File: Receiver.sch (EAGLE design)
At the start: 11 parts, among them IC1 25LC080P, J1 PIC_ICSP_6_PIN, U1 915MHz, U2 DS3234, X1 BU-SMA-V

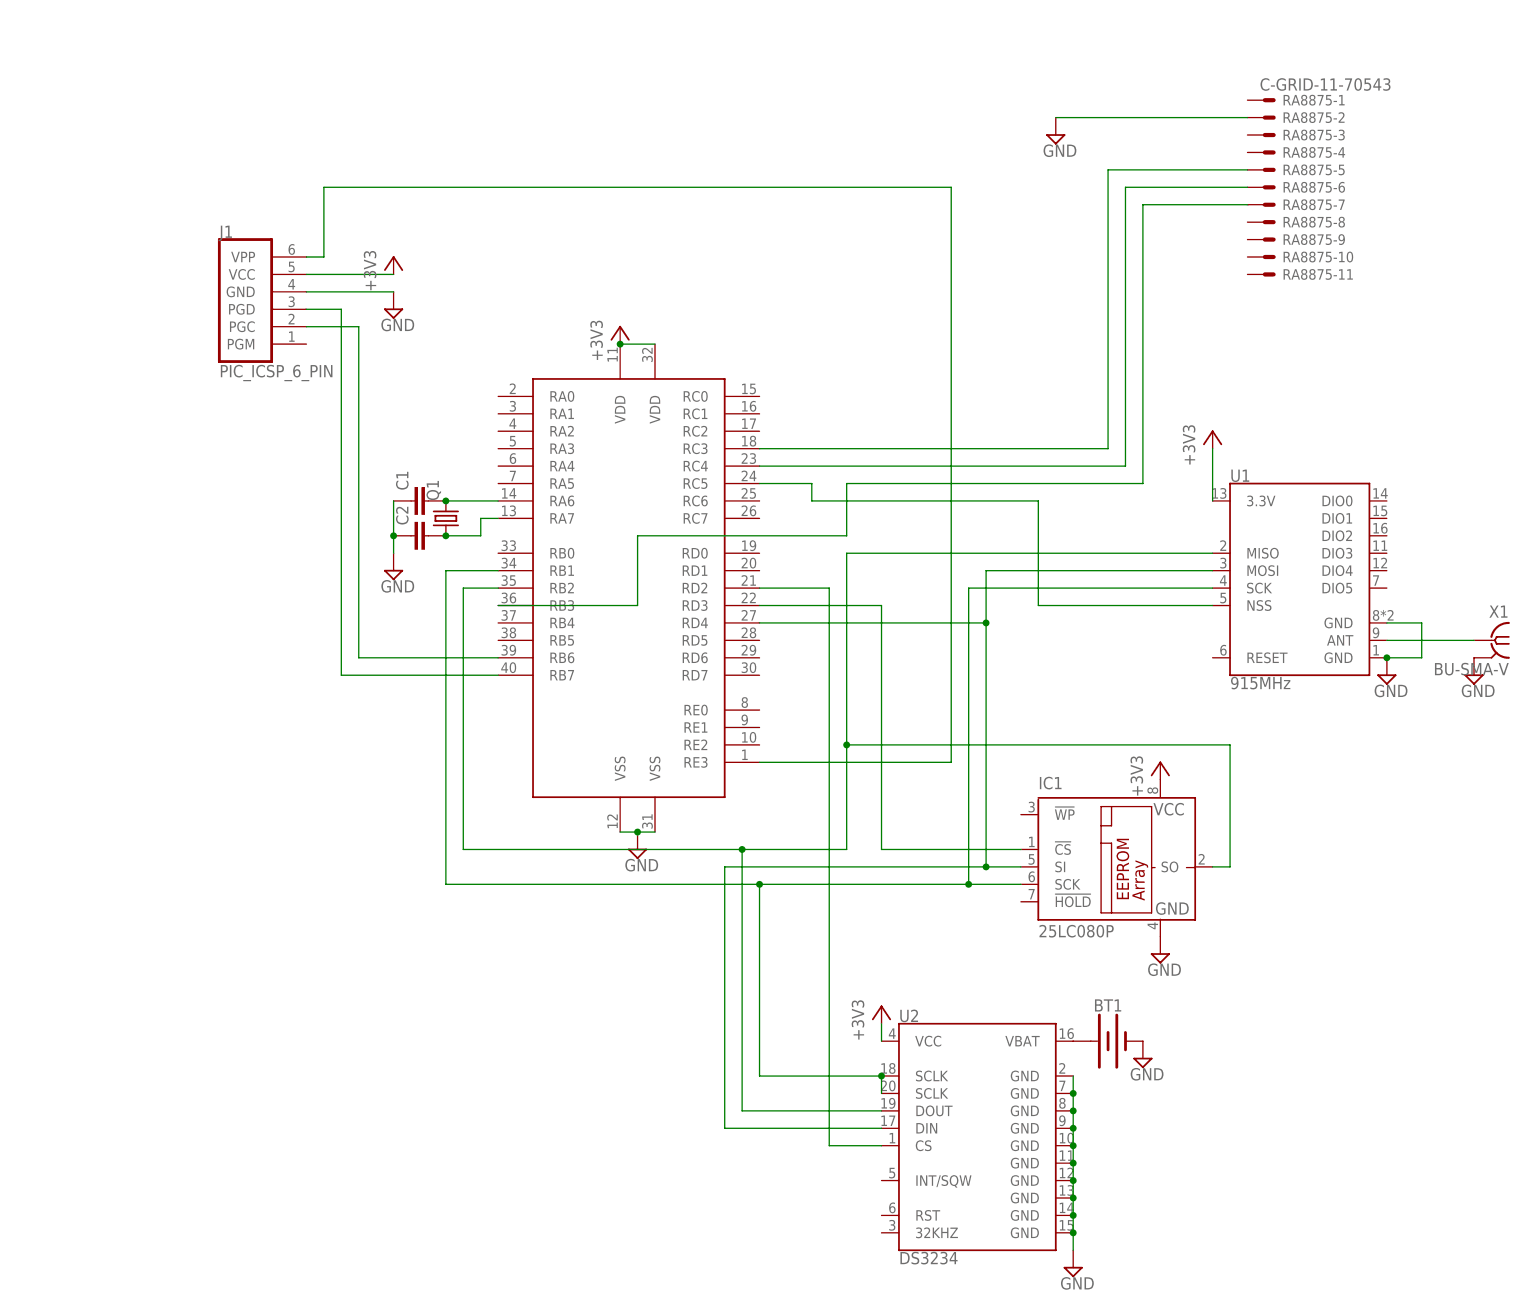
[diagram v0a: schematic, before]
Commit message: Updates
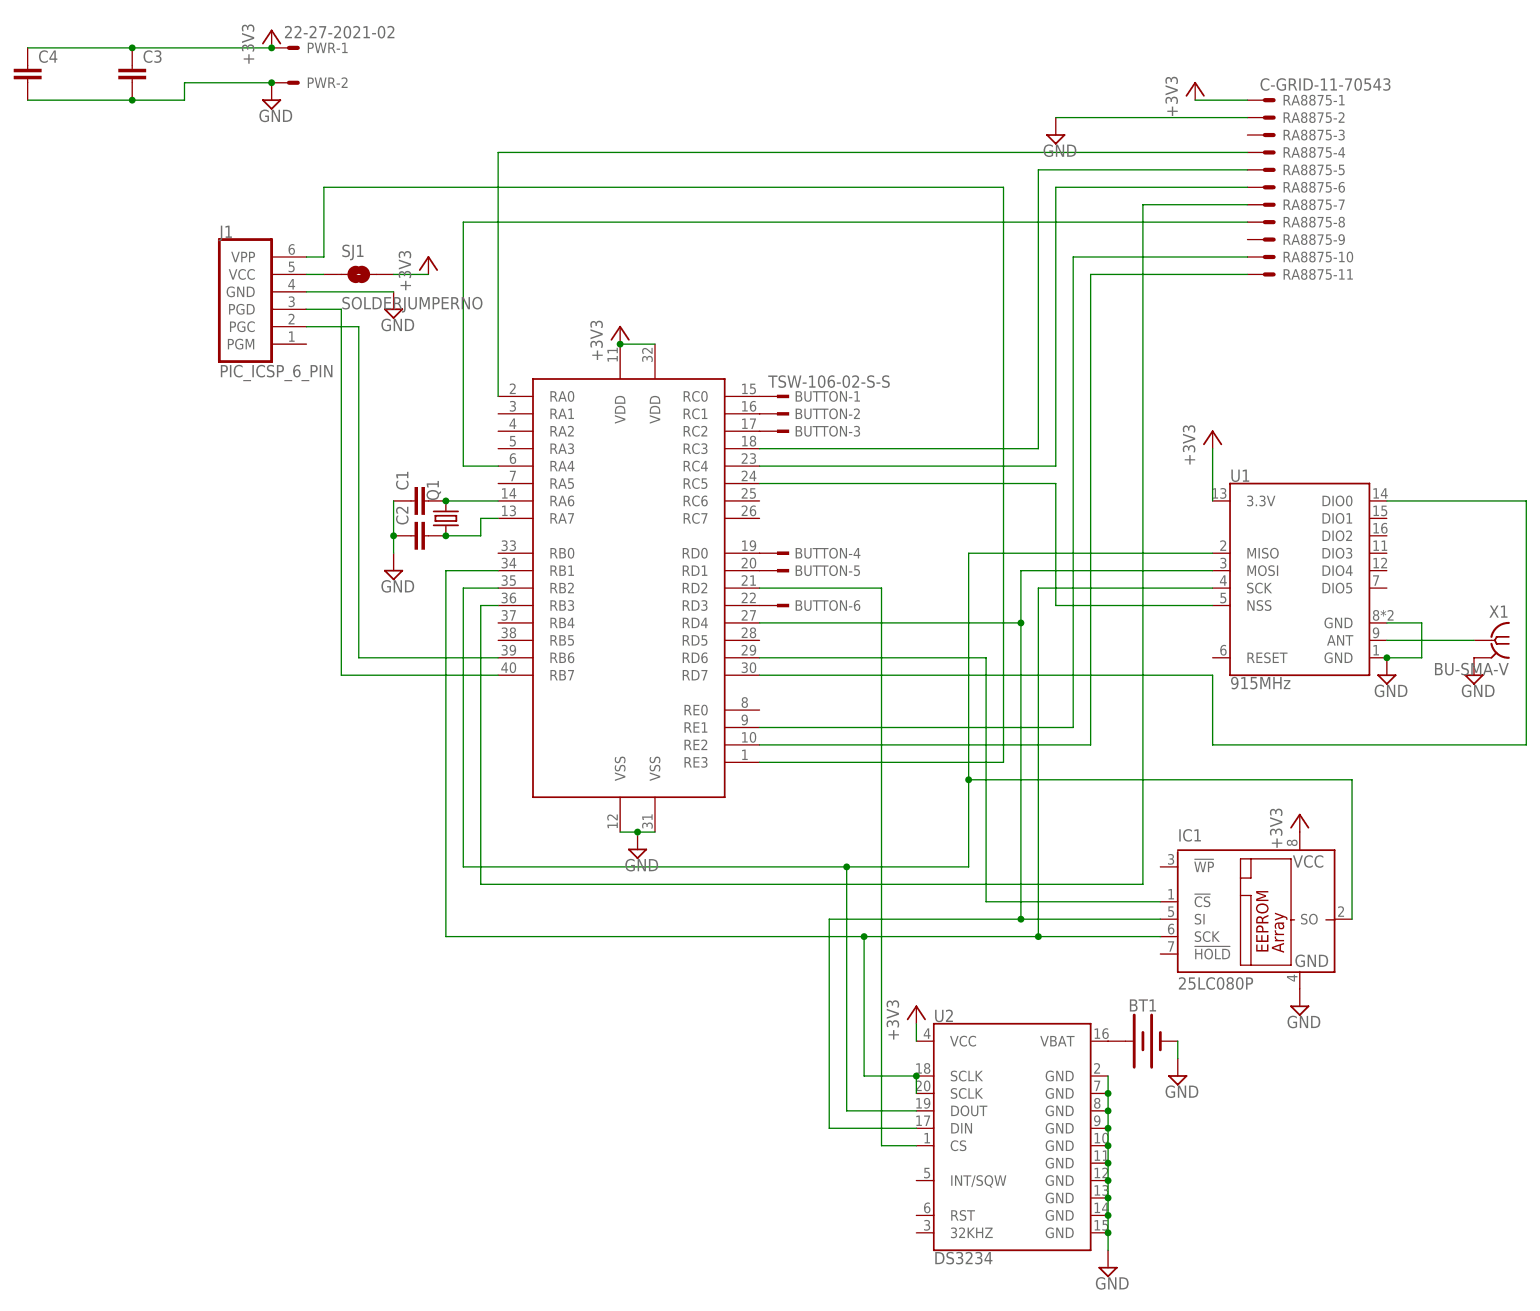
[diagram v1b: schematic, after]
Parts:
- added BUTTON: TSW-106-02-S-S, con-samtec:TSW-106-02-S-S
- added C3, C4: (no value), resistor:C-EU050-025X075
- added PWR: 22-27-2021-02, con-molex:22-27-2021-02
- added SJ1: SOLDERJUMPERNO, SparkFun-Retired:SOLDERJUMPERNO
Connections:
- net N$10 renamed MOSI1
- net N$11 renamed MOSI2
- net N$6 renamed SCK1
- net N$7 renamed MISO1
- net N$8 renamed SCK2
- net N$9 renamed MISO2
- new net N$10: BUTTON-4.1, U$1.RD0
- new net N$11: BUTTON-6.1, U$1.RD3
- new net N$17: RA8875-8.S, U$1.RA4
- new net N$18: RA8875-4.S, U$1.RA0
- new net N$19: RA8875-10.S, U$1.RE1
- new net N$20: RA8875-11.S, U$1.RE2
- new net N$21: U$1.RD7, U1.DIO0
- new net N$22: J1.VCC, SJ1.1
- new net N$6: BUTTON-1.1, U$1.RC0
- new net N$7: BUTTON-2.1, U$1.RC1
- new net N$8: BUTTON-3.1, U$1.RC2
- new net N$9: BUTTON-5.1, U$1.RD1
- net +3V3: now also C3.1, C4.1, PWR-1.S, RA8875-1.S, SJ1.2; no longer J1.VCC
- net GND: now also C3.2, C4.2, PWR-2.S
- net N$12: now also U$1.RD6; no longer U$1.RD3
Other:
- moved on the sheet: BT1, IC1, U2
